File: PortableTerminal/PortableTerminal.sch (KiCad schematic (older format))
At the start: 56 parts, among them J1 Barrel_Jack, J10 RCAJack, J11 Conn_01x02, J2 Conn_01x01, J3 Conn_01x01, J4 ICSP, J5 Conn_01x01, J6 Conn_01x01, J7 Conn_01x04, J8 Conn_01x04, J9 RCAJack, P1 Mini-DIN_6pins_ver4, Q1 2N3904, Q2 2N3904, SW1 SW_Push, U1 LM7805_TO220, U2 ATMEGA328P-PU, U3 LCD-016N002L, U4 MicroSD_SPI_CD, Y1 Crystal

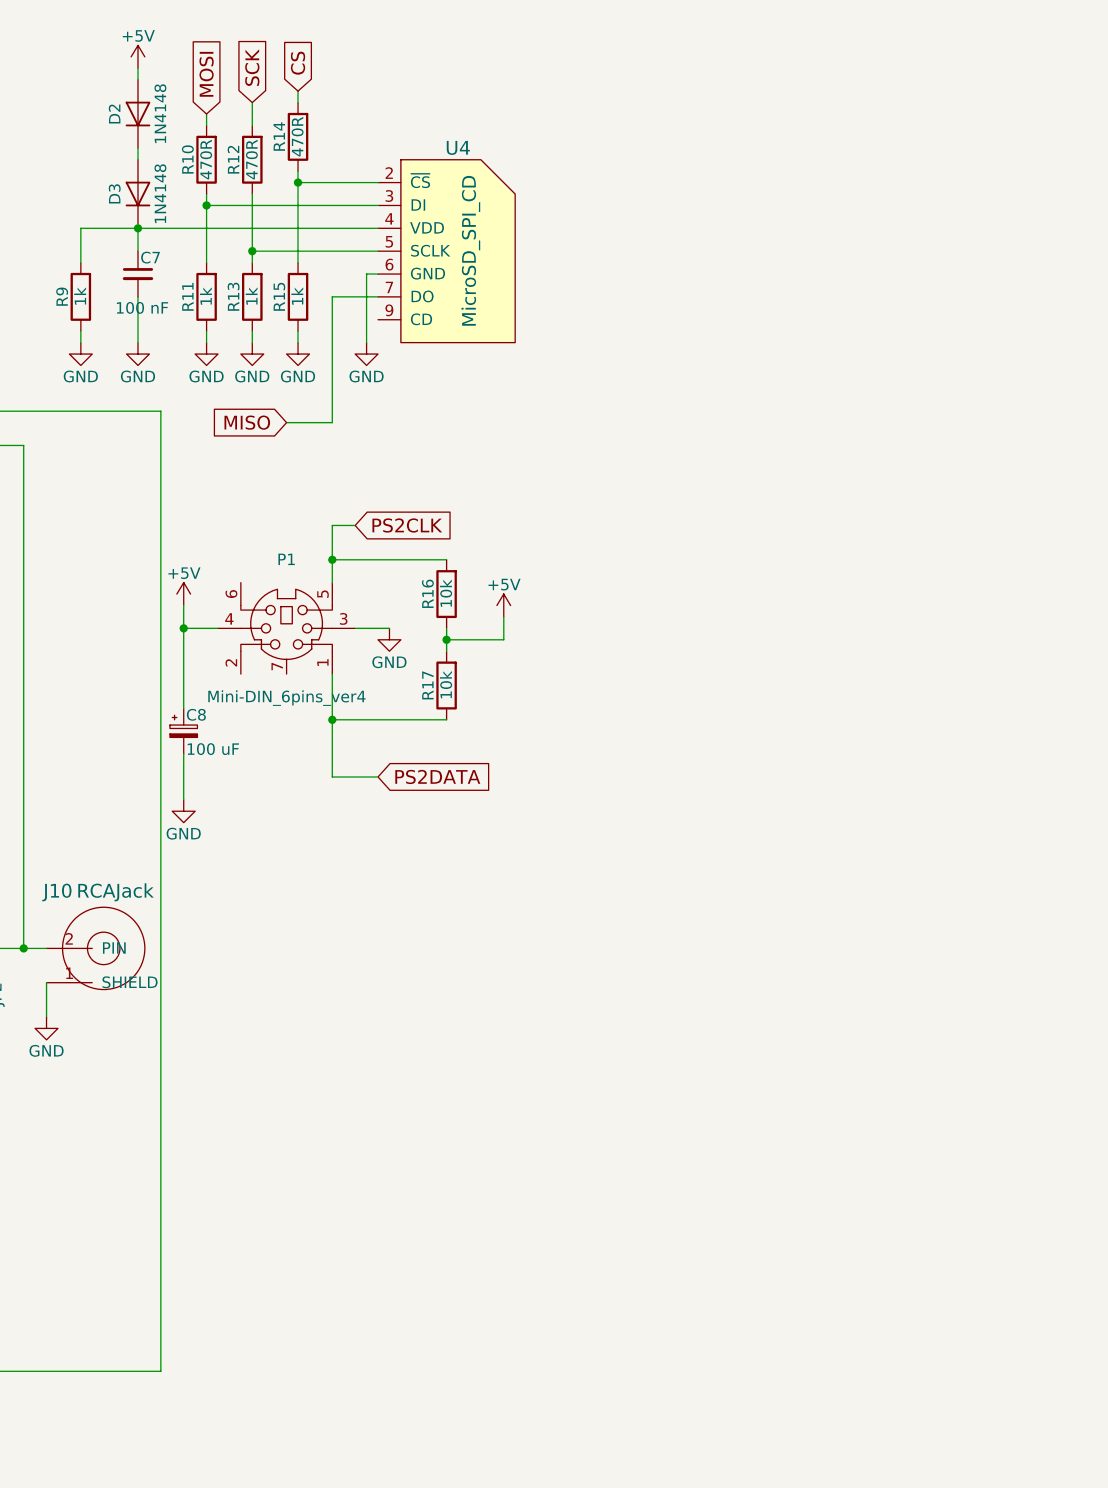
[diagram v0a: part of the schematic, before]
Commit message: Added frequency counter and power measurement circuitry to PortableTerminal
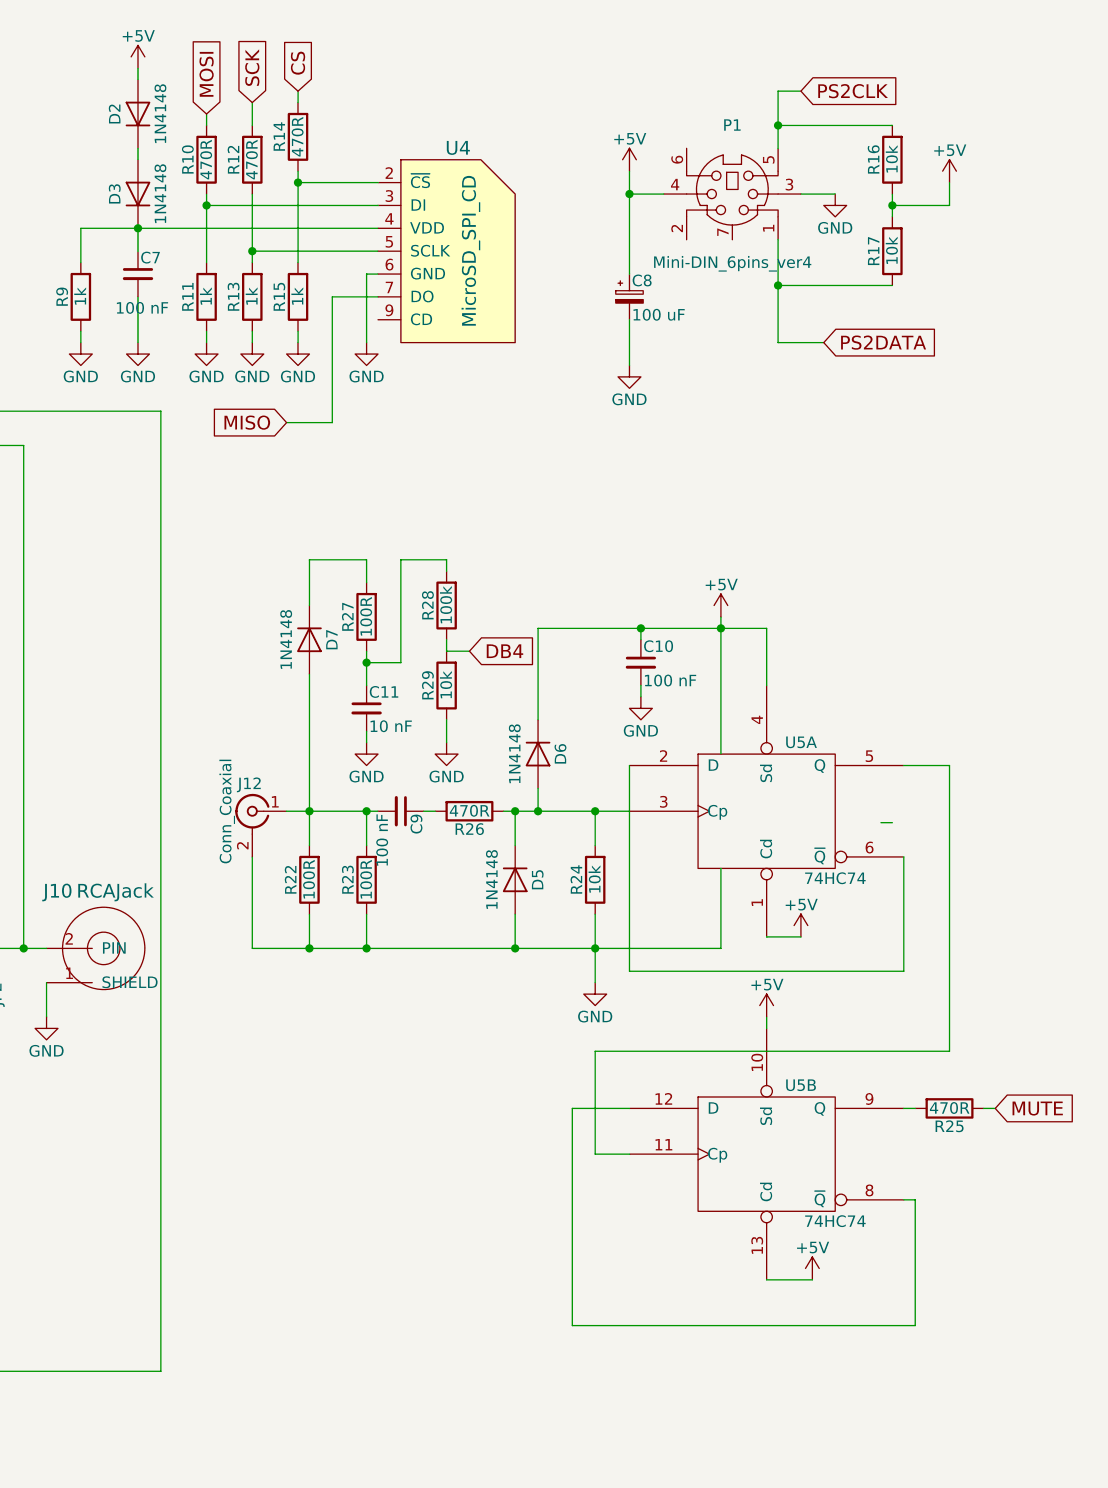
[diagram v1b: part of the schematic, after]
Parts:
- added C10, C9: 100 nF, Capacitors_THT:C_Disc_D5.0mm_W2.5mm_P2.50mm, symbol C_Small
- added C11: 10 nF, Capacitors_THT:C_Disc_D5.0mm_W2.5mm_P2.50mm, symbol C_Small
- added D5, D6, D7: 1N4148, Diodes_THT:D_DO-35_SOD27_P7.62mm_Horizontal, symbol D
- added J12: Conn_Coaxial, PortableTerminal:bnc_90_1-1337543-0_pad_combo, symbol Conn_Coaxial
- added R22, R23: 100R, Resistors_THT:R_Axial_DIN0309_L9.0mm_D3.2mm_P12.70mm_Horizontal, symbol R
- added R24, R29: 10k, Resistors_THT:R_Axial_DIN0207_L6.3mm_D2.5mm_P7.62mm_Horizontal, symbol R
- added R25, R26: 470R, Resistors_THT:R_Axial_DIN0207_L6.3mm_D2.5mm_P7.62mm_Horizontal, symbol R
- added R27: 100R, Resistors_THT:R_Axial_DIN0207_L6.3mm_D2.5mm_P7.62mm_Horizontal, symbol R
- added R28: 100k, Resistors_THT:R_Axial_DIN0207_L6.3mm_D2.5mm_P7.62mm_Horizontal, symbol R
- added U5: 74HC74, Housings_DIP:DIP-14_W7.62mm_Socket, symbol 74HC74
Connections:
- net +5V: now also C10.1, D6.1 (K), U5.1 (Cd), U5.10 (Sd), U5.13 (Cd), U5.14 (VCC), U5.14 (VCC), U5.4 (Sd)
- net DB4: now also R28.1, R29.2
- net GND: now also C10.2, C11.2, D5.2 (A), J12.2 (Ext), R22.1, R23.1, R24.1, R29.1, U5.7 (GND), U5.7 (GND)
- net MUTE: now also R25.1
- new net: D5.1 (K), D6.2 (A), R24.2, R26.1, U5.3 (Cp)
- new net: C9.1, R26.2
- new net: R25.2, U5.9 (Q)
- new net: C9.2, D7.2 (A), J12.1 (In), R22.2, R23.2
- new net: D7.1 (K), R27.2
- new net: C11.1, R27.1, R28.2
- new net: U5.2 (D), U5.6 (~Q)
- new net: U5.11 (Cp), U5.5 (Q)
- new net: U5.12 (D), U5.8 (~Q)
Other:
- moved on the sheet: C8, P1, R16, R17

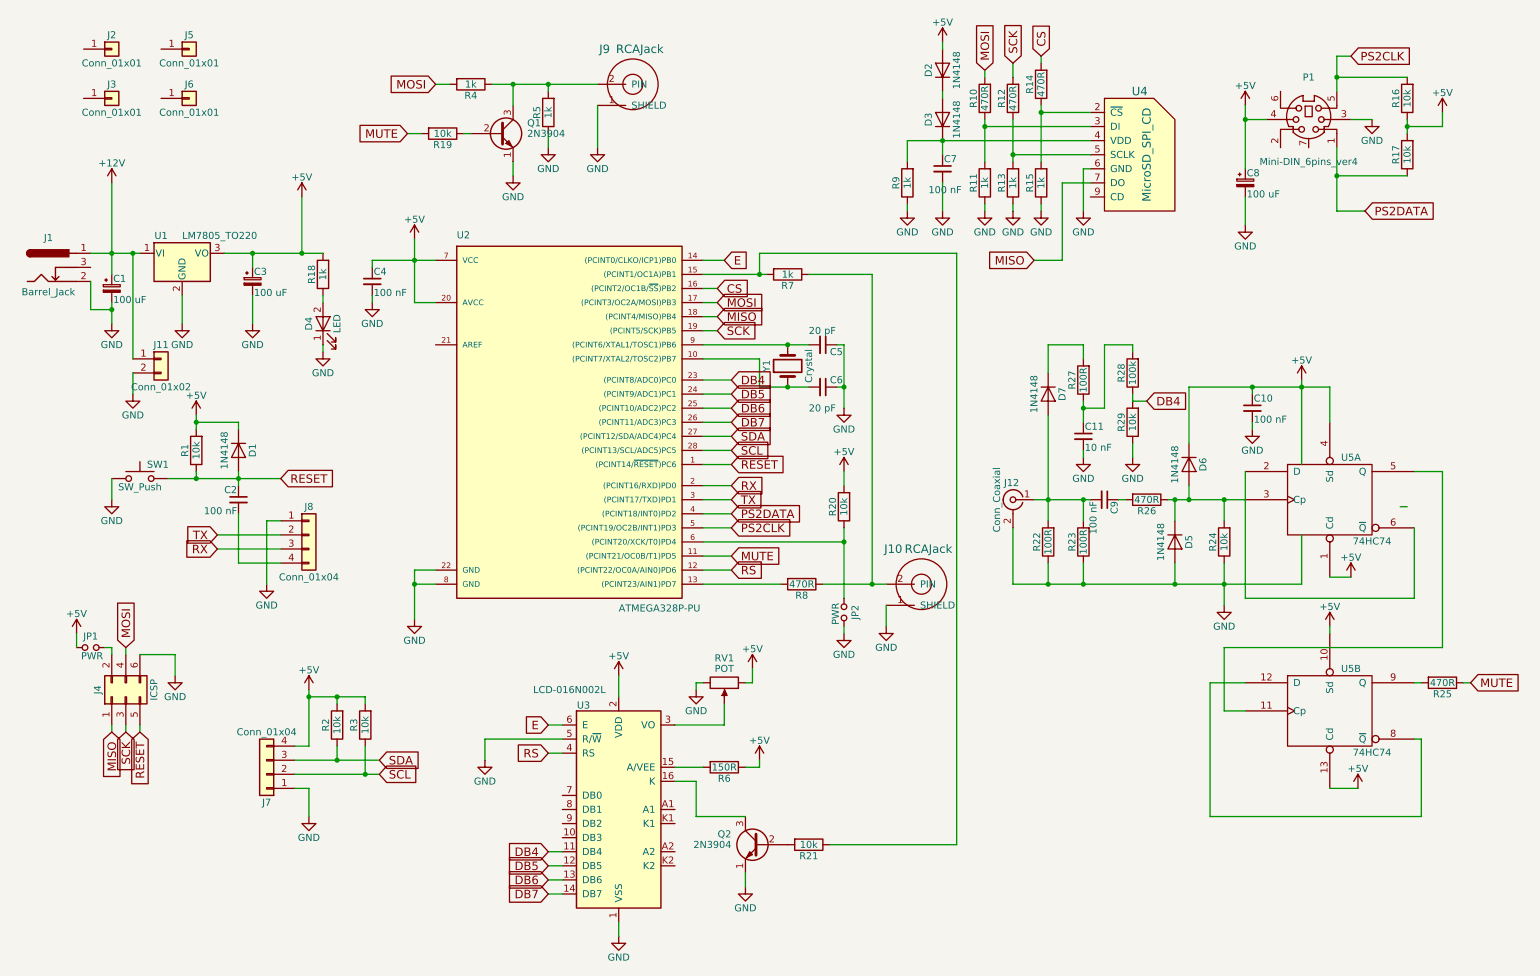
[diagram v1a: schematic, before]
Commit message: Added common mode choke to PortableTerminal
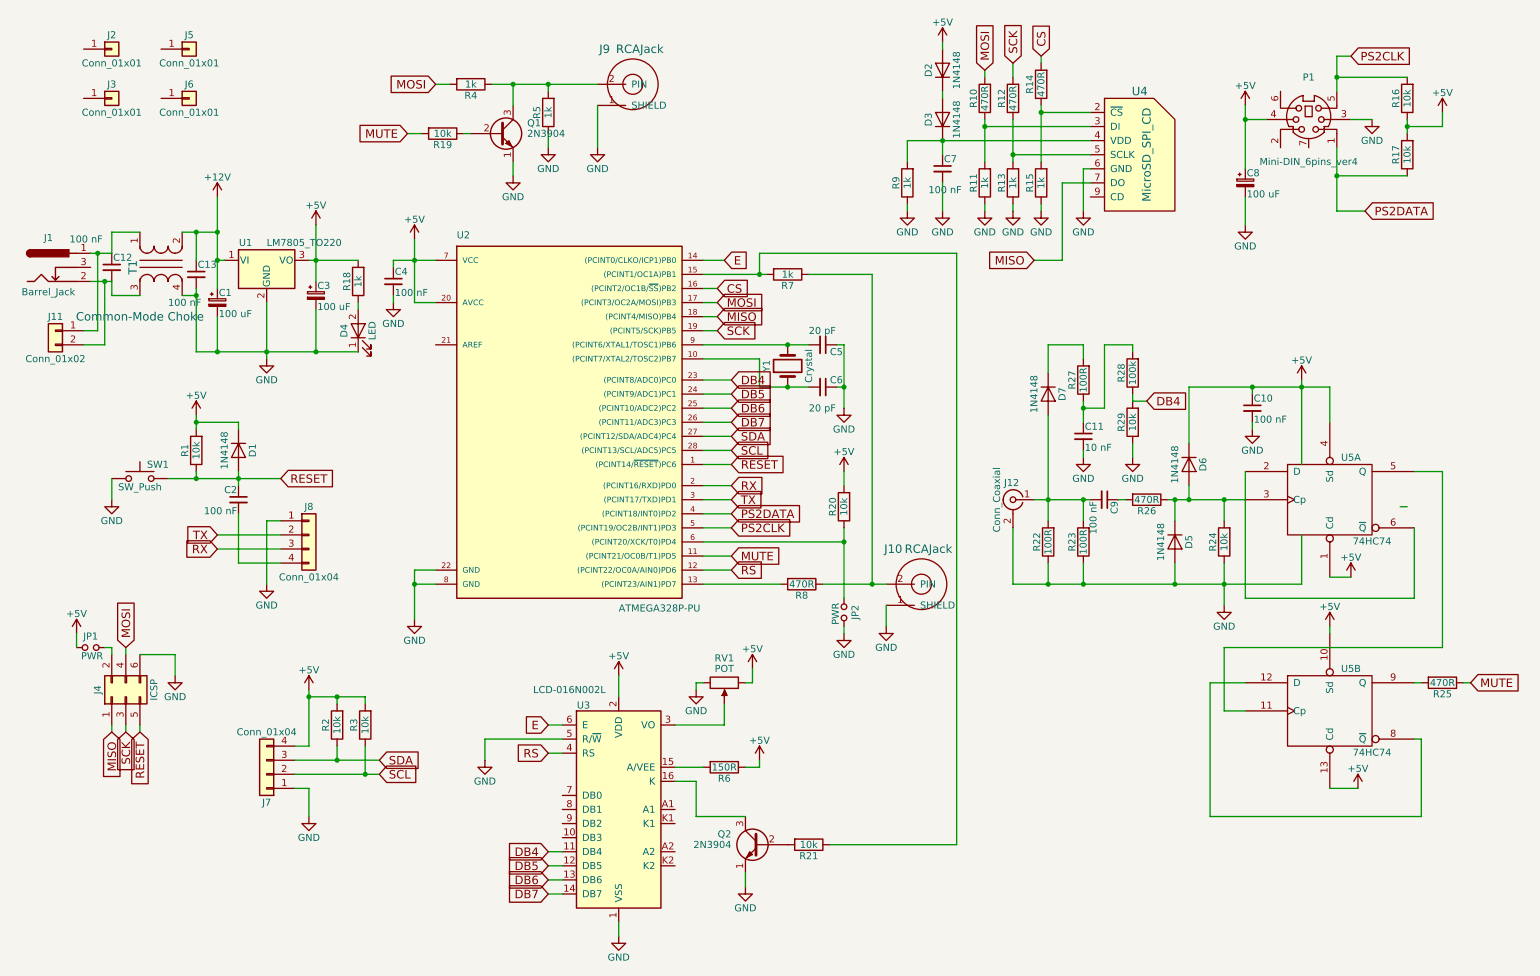
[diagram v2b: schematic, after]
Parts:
- added C12, C13: 100 nF, Capacitors_THT:C_Disc_D5.0mm_W2.5mm_P2.50mm, symbol C_Small
- added T1: Common-Mode Choke, PortableTerminal:DoubleWindingTransformer, symbol DoubleWindingTransformer
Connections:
- net +12V: now also C13.1, T1.2; no longer J1.1, J11.1 (Pin_1)
- net GND: now also C13.2, T1.4; no longer J1.2, J11.2 (Pin_2)
- new net: C12.1, J1.1, J11.1 (Pin_1), T1.1
- new net: C12.2, J1.2, J11.2 (Pin_2), T1.3
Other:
- moved on the sheet: C1, C3, C4, D4, J11, R18, U1
